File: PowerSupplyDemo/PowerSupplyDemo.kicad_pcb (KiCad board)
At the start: 8 copper layers, 137 parts, among them J1 USB_C, Q1 BSZ060NE2LSATMA1, Q2 BSZ060NE2LSATMA1, SW1 219-3LPSTR, SW2 219-7LPSTR, SW3 219-2LPST, U2 TVS2200DRV, U3 TPS65988DJ, U4 LTC3833IUDC, U5 CP2102N-A01-GQFN28, U6 TPS6591286YFFR

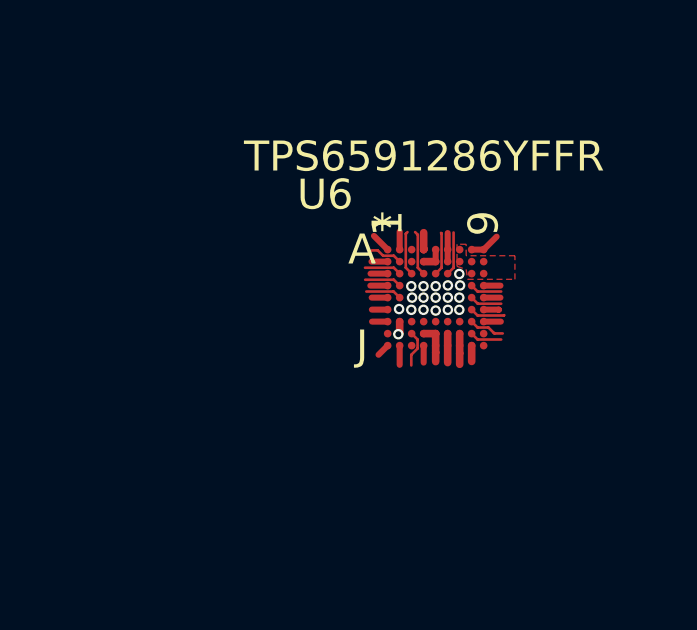
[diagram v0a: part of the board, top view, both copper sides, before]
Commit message: updated constraints again.
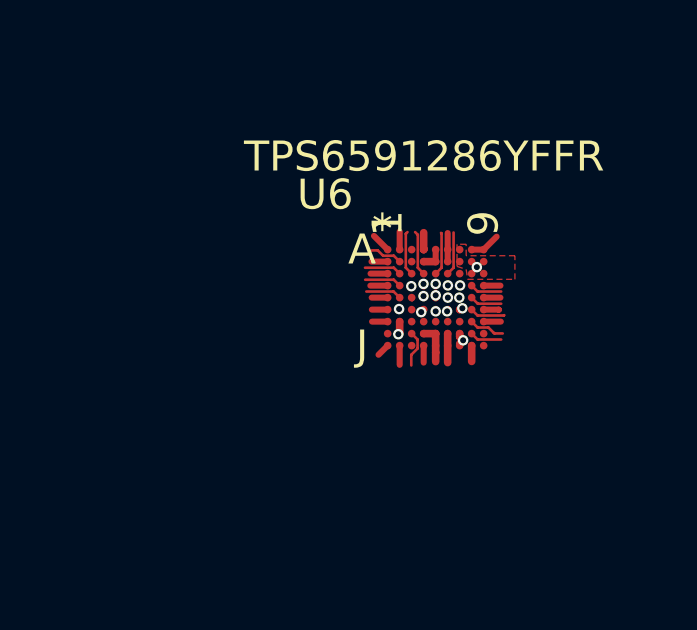
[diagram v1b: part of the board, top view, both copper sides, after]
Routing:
- net I2C0_SCL_C0: track 0.00 -> 2.72 mm
- net I2C0_SDA_C0: track 0.00 -> 2.37 mm
- net DCD1_PWM_AVS: track 0.00 -> 2.06 mm
- net DCD1_CLK_AVS: track 0.00 -> 1.96 mm
- net WATCHDOG_CLOCK_OUT: track 0.00 -> 1.96 mm
- net SPI0_D1_C0: track 0.00 -> 1.87 mm
- net SPI0_CLK_C0: track 0.00 -> 1.86 mm
- net SPI0_D0_C0: track 0.00 -> 1.85 mm
- net PMIC_ENABLE: track 0.00 -> 1.79 mm
- net /PMIC/LDOA: track 0.00 -> 1.78 mm
- net /PMIC/POS_1P8_IO: track 0.43 -> 1.92 mm
- net /PMIC/iic_or_spi_cntrl: track 0.00 -> 1.40 mm
- net POS1P8_C0: track 0.00 -> 1.35 mm
- net POS3P3_C0: track 0.00 -> 1.02 mm
- net VSYS_3P3: track 2.08 -> 2.47 mm, vias 1 -> 3
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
